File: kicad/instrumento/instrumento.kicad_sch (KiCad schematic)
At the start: 4 parts, among them U1 Teensy4.1, U2 Teensy4.0_AudioShield_REVD

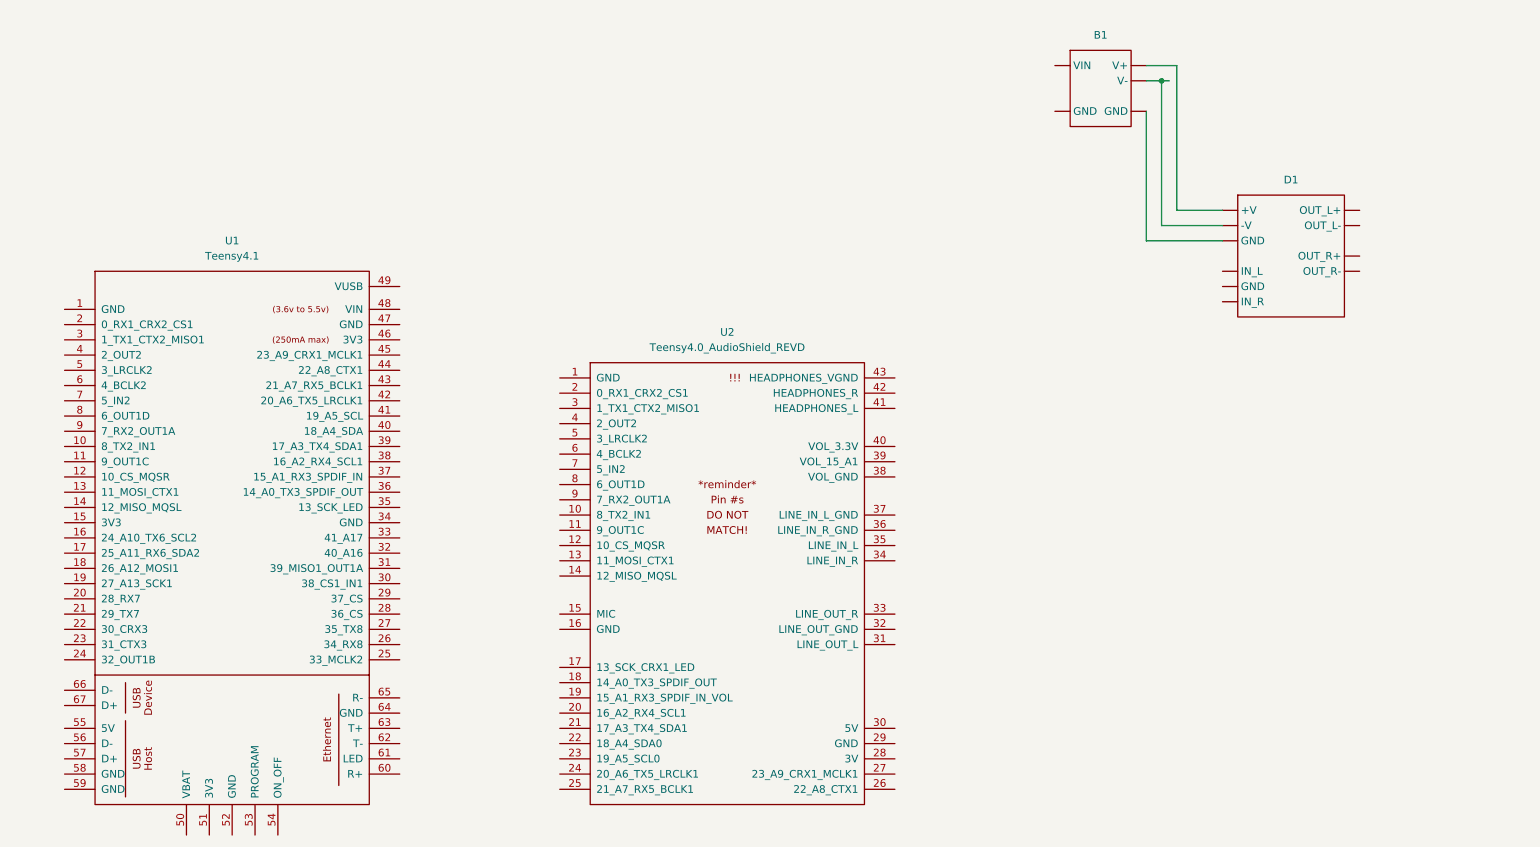
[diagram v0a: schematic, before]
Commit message: Audio output
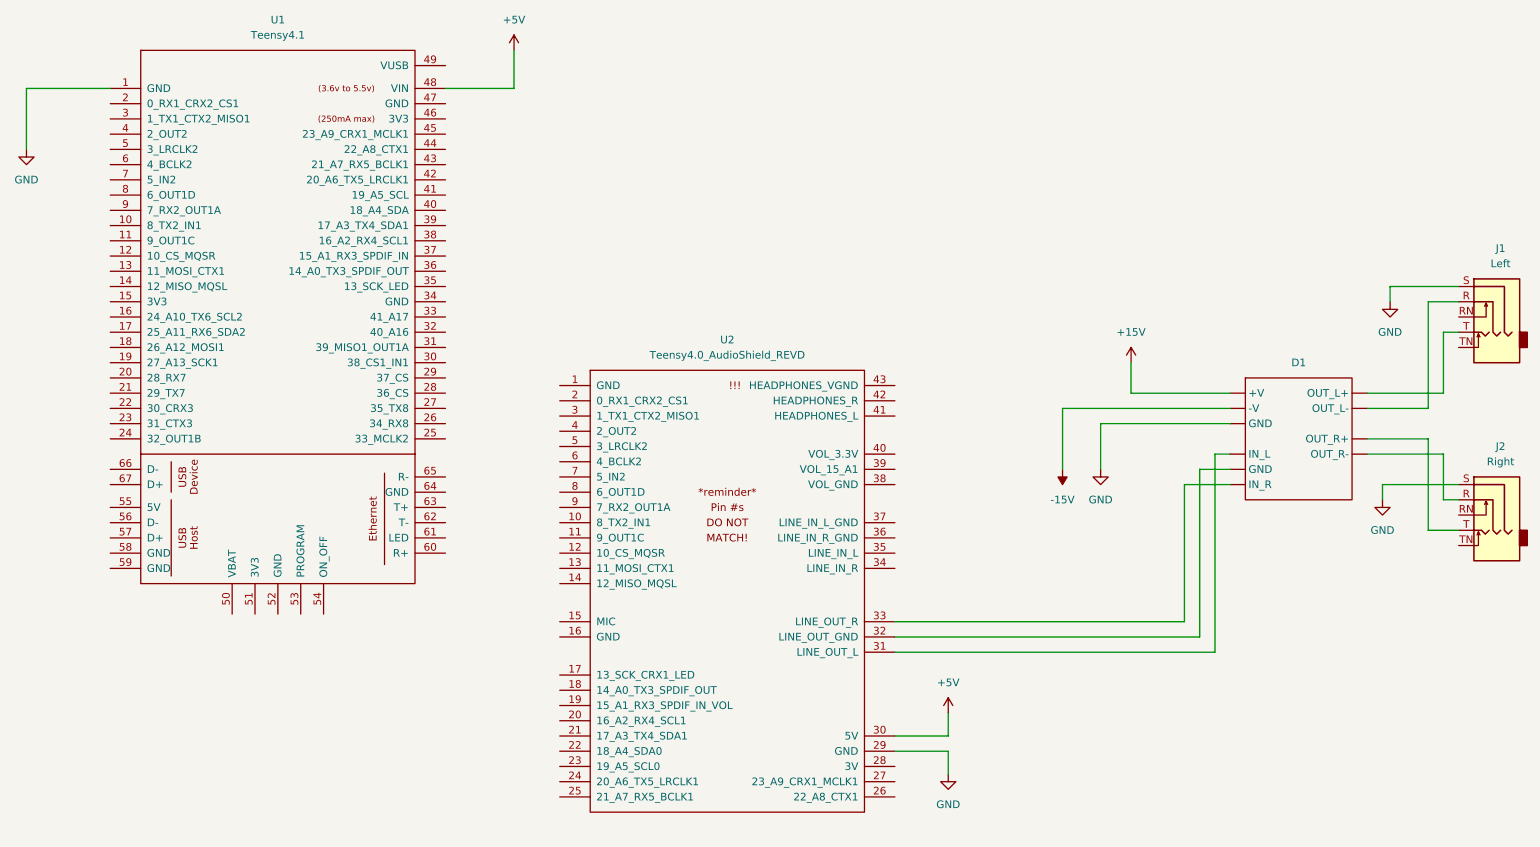
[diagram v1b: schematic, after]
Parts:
- removed B1: (no value), symbol parts:20_Symmetric_Boost
- added J1: Left, symbol Connector_Audio:AudioJack3_SwitchTR
- added J2: Right, symbol Connector_Audio:AudioJack3_SwitchTR
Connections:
- net GND: now reaches U1.1 (GND)
- net GND: now also D1. (OUT_R-), U2.29 (GND), J1.S, J2.S
- net +5V: now reaches U1.48 (VIN)
- net +5V: now also U2.30 (5V)
- net at U2.31 (LINE_OUT_L): now also D1. (OUT_R-)
- net at U2.32 (LINE_OUT_GND): now also D1. (OUT_R-)
- net at U2.33 (LINE_OUT_R): now also D1. (OUT_R-)
- new net: D1. (OUT_R-), J2.R
- new net: D1. (OUT_R-), J2.T
- new net: D1. (OUT_R-), J1.R
- new net: D1. (OUT_R-), J1.T
- new net +15V: D1. (OUT_R-)
- new net -15V: D1. (OUT_R-)
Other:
- moved on the sheet: D1, U1, U2
